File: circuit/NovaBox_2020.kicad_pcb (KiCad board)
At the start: 2 copper layers, 82 x 30 mm, 87 parts, among them P1 MH, P2 MH, P3 MH, P4 MH, P5 USB, Q1 MMBT3904, Q2 IRLML6344, Q3 IRLML6401, Q4 MMBT3904, Q5 MMBT3904, SW1 PIO18, SW2 PIO21, SW3 PIO8, SW4 PIO0, SW5 PIO1, SW6 ON/OFF, U1 MCP6004, U2 CSR8635_MODULE, U3 CSR_DebugSmall, U4 PAM8304, U5 PAM8304, U6 LT1308

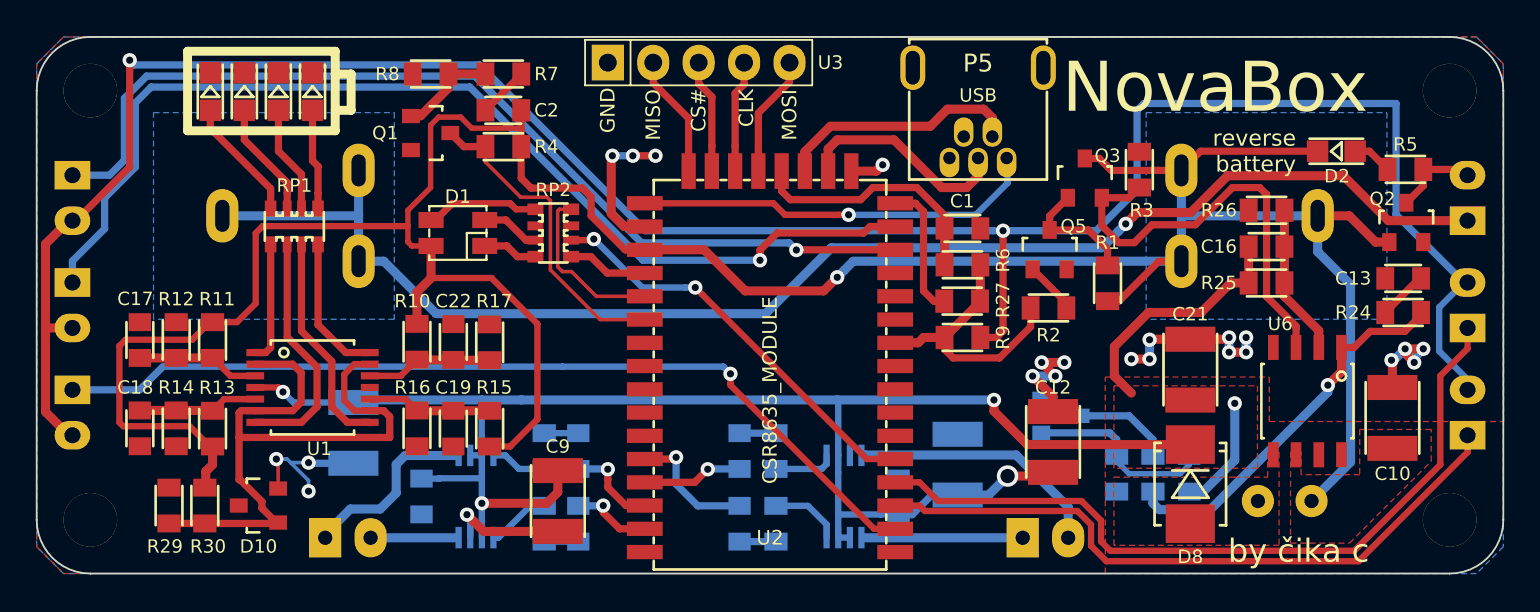
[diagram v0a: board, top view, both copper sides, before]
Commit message: NovaBox 2020 update
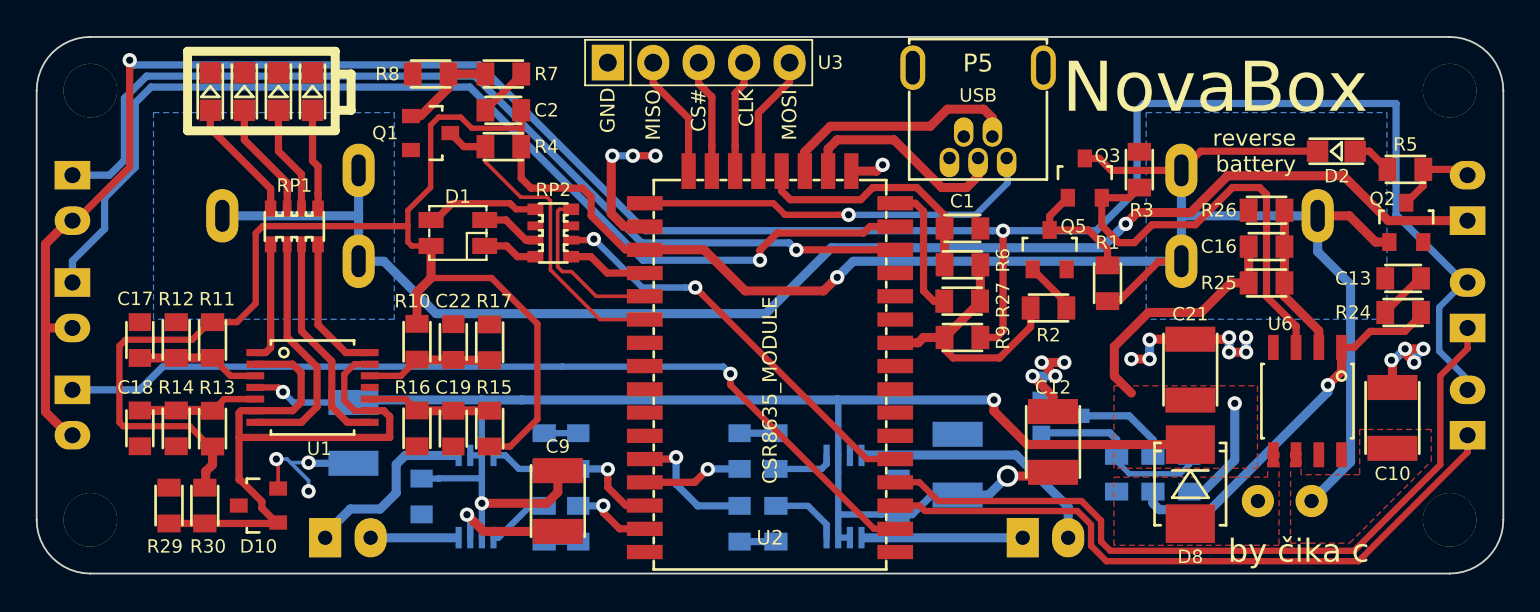
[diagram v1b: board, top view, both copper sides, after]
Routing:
- removed copper zone on B.Cu, net GND
- removed copper zone on F.Cu, net GND
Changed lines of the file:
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@@
-(kicad_pcb (version 20171130) (host pcbnew "(5.0.0)")
+(kicad_pcb (version 20171130) (host pcbnew "(5.1.4)-1")
   (general
     (thickness 1.6)
@@
   )
   (setup
-    (last_trace_width 0.4064)
+    (last_trace_width 0.2032)
     (user_trace_width 0.254)
     (user_trace_width 0.3048)
@@
     (zone_45_only yes)
     (trace_min 0.2)
-    (segment_width 0.5)
-    (edge_width 0.1)
     (via_size 0.8)
     (via_drill 0.4)
@@
     (uvia_min_size 0.2)
     (uvia_min_drill 0.1)
+    (edge_width 0.1)
+    (segment_width 0.5)
     (pcb_text_width 0.3)
     (pcb_text_size 1.5 1.5)
@@
     (add_net VR_SHDN)
   )
+  (module NovaBox:MountingHole (layer F.Cu)
+    (at 62 53)
+    (descr "Mounting hole")
+    (tags "Mounting hole")
+    (fp_text reference P4 (at 0 0.95) (layer F.SilkS) hide
+      (effects (font (size 0.127 0.127) (thickness 0.01)))
+    )
+    (fp_text value MH (at 0 -0.9) (layer F.SilkS) hide
+      (effects (font (size 0.127 0.127) (thickness 0.01)))
+    )
+    (fp_circle (center 0 0) (end 1.5 0) (layer F.CrtYd) (width 0.05))
+    (fp_circle (center 0 0) (end 3.1 0) (layer F.CrtYd) (width 0.05))
+    (fp_line (start 3.1 0) (end 1.55 -2.684) (layer F.CrtYd) (width 0.05))
+    (fp_line (start -1.55 -2.684) (end -3.1 0) (layer F.CrtYd) (width 0.05))
+    (fp_line (start 1.55 -2.684) (end -1.55 -2.684) (layer F.CrtYd) (width 0.05))
+    (fp_line (start 1.55 2.684) (end 3.1 0) (layer F.CrtYd) (width 0.05))
+    (fp_line (start -1.55 2.684) (end 1.55 2.684) (layer F.CrtYd) (width 0.05))
+    (fp_line (start -3.1 0) (end -1.55 2.684) (layer F.CrtYd) (width 0.05))
+    (pad 1 thru_hole circle (at 0 0) (size 3 3) (drill 3) (layers *.Cu *.Mask))
+  )
   (module NovaBox:COIL0608 (layer B.Cu)
     (at 128.778 75.946 180)
@@
     (pad 1 thru_hole circle (at 0 0) (size 3 3) (drill 3) (layers *.Cu *.Mask))
   )
-  (module NovaBox:MountingHole (layer F.Cu)
-    (at 62 53)
-    (descr "Mounting hole")
-    (tags "Mounting hole")
-    (fp_text reference P4 (at 0 0.95) (layer F.SilkS) hide
-      (effects (font (size 0.127 0.127) (thickness 0.01)))
-    )
-    (fp_text value MH (at 0 -0.9) (layer F.SilkS) hide
-      (effects (font (size 0.127 0.127) (thickness 0.01)))
-    )
-    (fp_circle (center 0 0) (end 1.5 0) (layer F.CrtYd) (width 0.05))
-    (fp_circle (center 0 0) (end 3.1 0) (layer F.CrtYd) (width 0.05))
-    (fp_line (start 3.1 0) (end 1.55 -2.684) (layer F.CrtYd) (width 0.05))
-    (fp_line (start -1.55 -2.684) (end -3.1 0) (layer F.CrtYd) (width 0.05))
-    (fp_line (start 1.55 -2.684) (end -1.55 -2.684) (layer F.CrtYd) (width 0.05))
-    (fp_line (start 1.55 2.684) (end 3.1 0) (layer F.CrtYd) (width 0.05))
-    (fp_line (start -1.55 2.684) (end 1.55 2.684) (layer F.CrtYd) (width 0.05))
-    (fp_line (start -3.1 0) (end -1.55 2.684) (layer F.CrtYd) (width 0.05))
-    (pad 1 thru_hole circle (at 0 0) (size 3 3) (drill 3) (layers *.Cu *.Mask))
-  )
   (module NovaBox:USB_MiniB_THT (layer F.Cu)
     (at 111.633 56.769 270)
@@
     )
   )
-  (gr_text "reverse\nbattery" (at 129.413 56.388) (layer F.SilkS)
-    (effects (font (size 0.9 0.9) (thickness 0.127)) (justify right))
-  )
   (gr_text https://github.com/nodep/NovaBox (at 100 66.548) (layer B.SilkS)
     (effects (font (size 1.5 1.5) (thickness 0.3)) (justify mirror))
   )
+  (gr_text "reverse\nbattery" (at 129.413 56.388) (layer F.SilkS)
+    (effects (font (size 0.9 0.9) (thickness 0.127)) (justify right))
+  )
   (gr_line (start 75.692 54.102) (end 76.581 54.102) (layer F.SilkS) (width 0.5))
   (gr_line (start 76.581 52.07) (end 75.692 52.07) (layer F.SilkS) (width 0.5))
@@
       )
     )
-  )
-  (zone (net 3) (net_name GND) (layer F.Cu) (hatch edge 0.508)
-    (connect_pads yes (clearance 0.254))
-    (min_thickness 0.254)
-    (fill yes (arc_segments 16) (thermal_gap 0.508) (thermal_bridge_width 0.508))
-    (polygon
-      (pts
-        (xy 118.75 80) (xy 118.745 69.0118) (xy 127.9144 69.0118) (xy 127.9144 71.501) (xy 141.0144 71.501)
-        (xy 141 51.5) (xy 139.5 50) (xy 60.5 50) (xy 59 51.5) (xy 59 78.5)
-        (xy 60.5 80)
-      )
-    )
-  )
-  (zone (net 3) (net_name GND) (layer B.Cu) (hatch edge 0.508)
-    (connect_pads yes (clearance 0.254))
-    (min_thickness 0.254)
-    (fill yes (arc_segments 16) (thermal_gap 0.508) (thermal_bridge_width 0.508))
-    (polygon
-      (pts
-        (xy 139.5 50) (xy 141 51.5) (xy 141 78.5) (xy 139.5 80) (xy 60.5 80)
-        (xy 59 78.5) (xy 59 51.5) (xy 60.5 50) (xy 129 50)
-      )
-    )
